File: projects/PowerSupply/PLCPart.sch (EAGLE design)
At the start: 31 parts, among them IC1 L7818CV, IC2 L7918CV, IC3 LM741P, IC4 LM741P, IC5 L7915CV, IC6 L7815CV, IC7 LM358N, IC8 LM358N, X1 MCU-PWR, X2 MCU-IN, X3 MCU-OUT

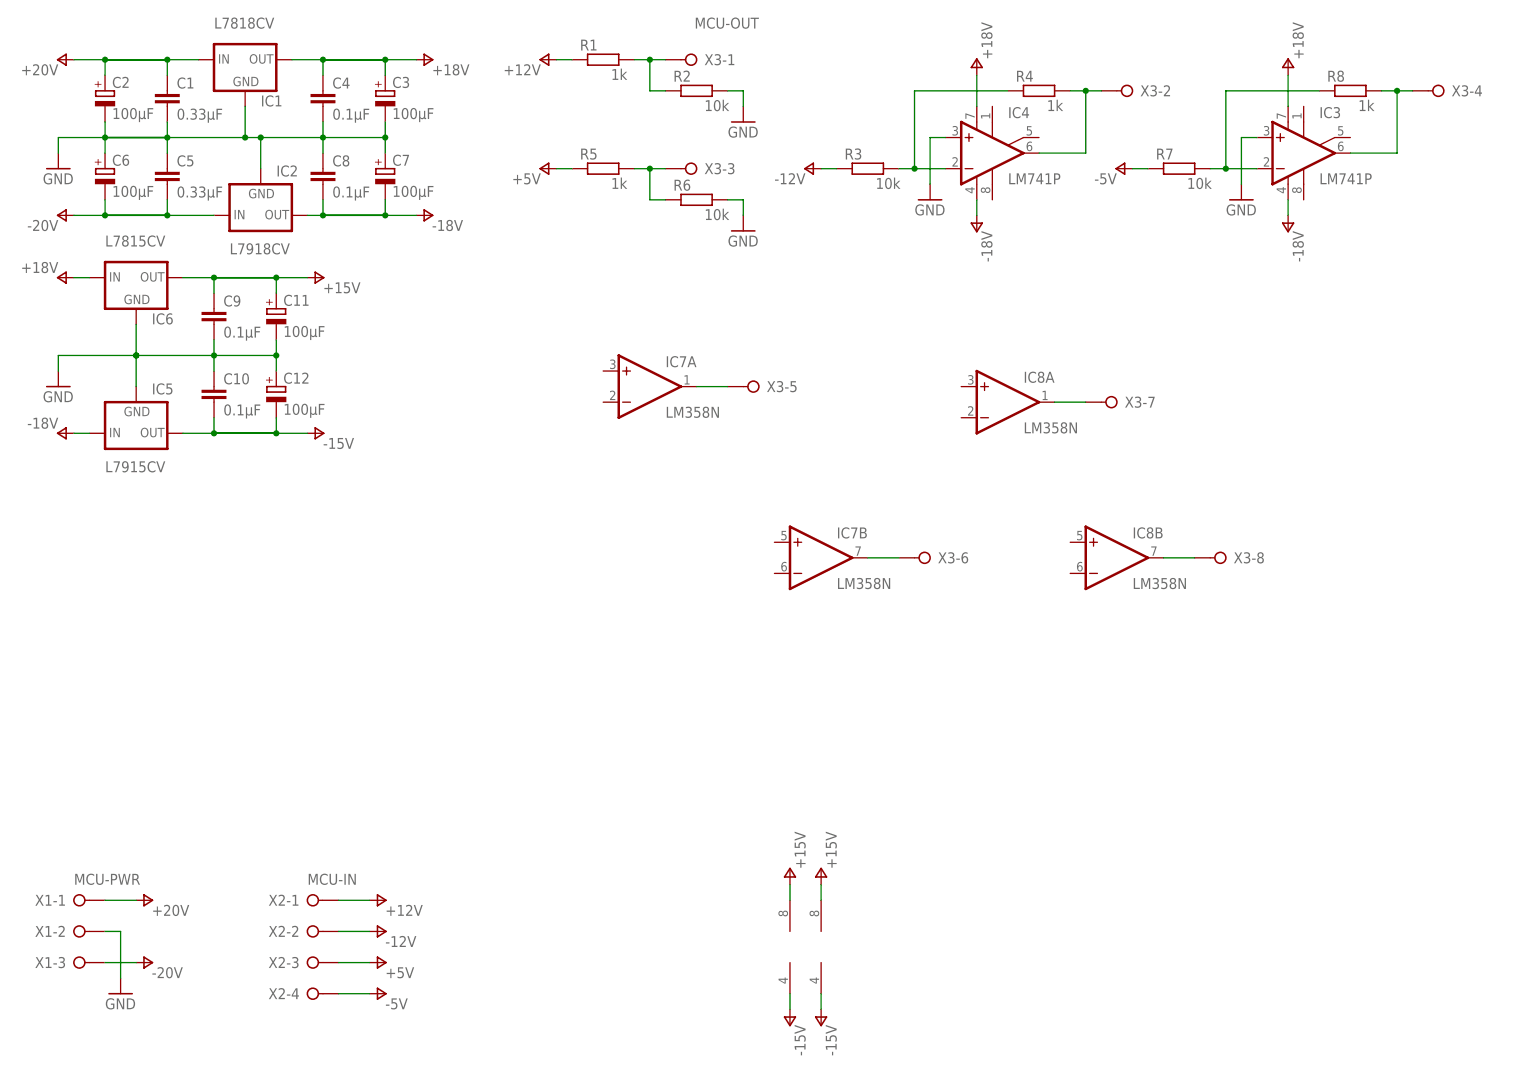
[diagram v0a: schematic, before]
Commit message: feat: plc part modified
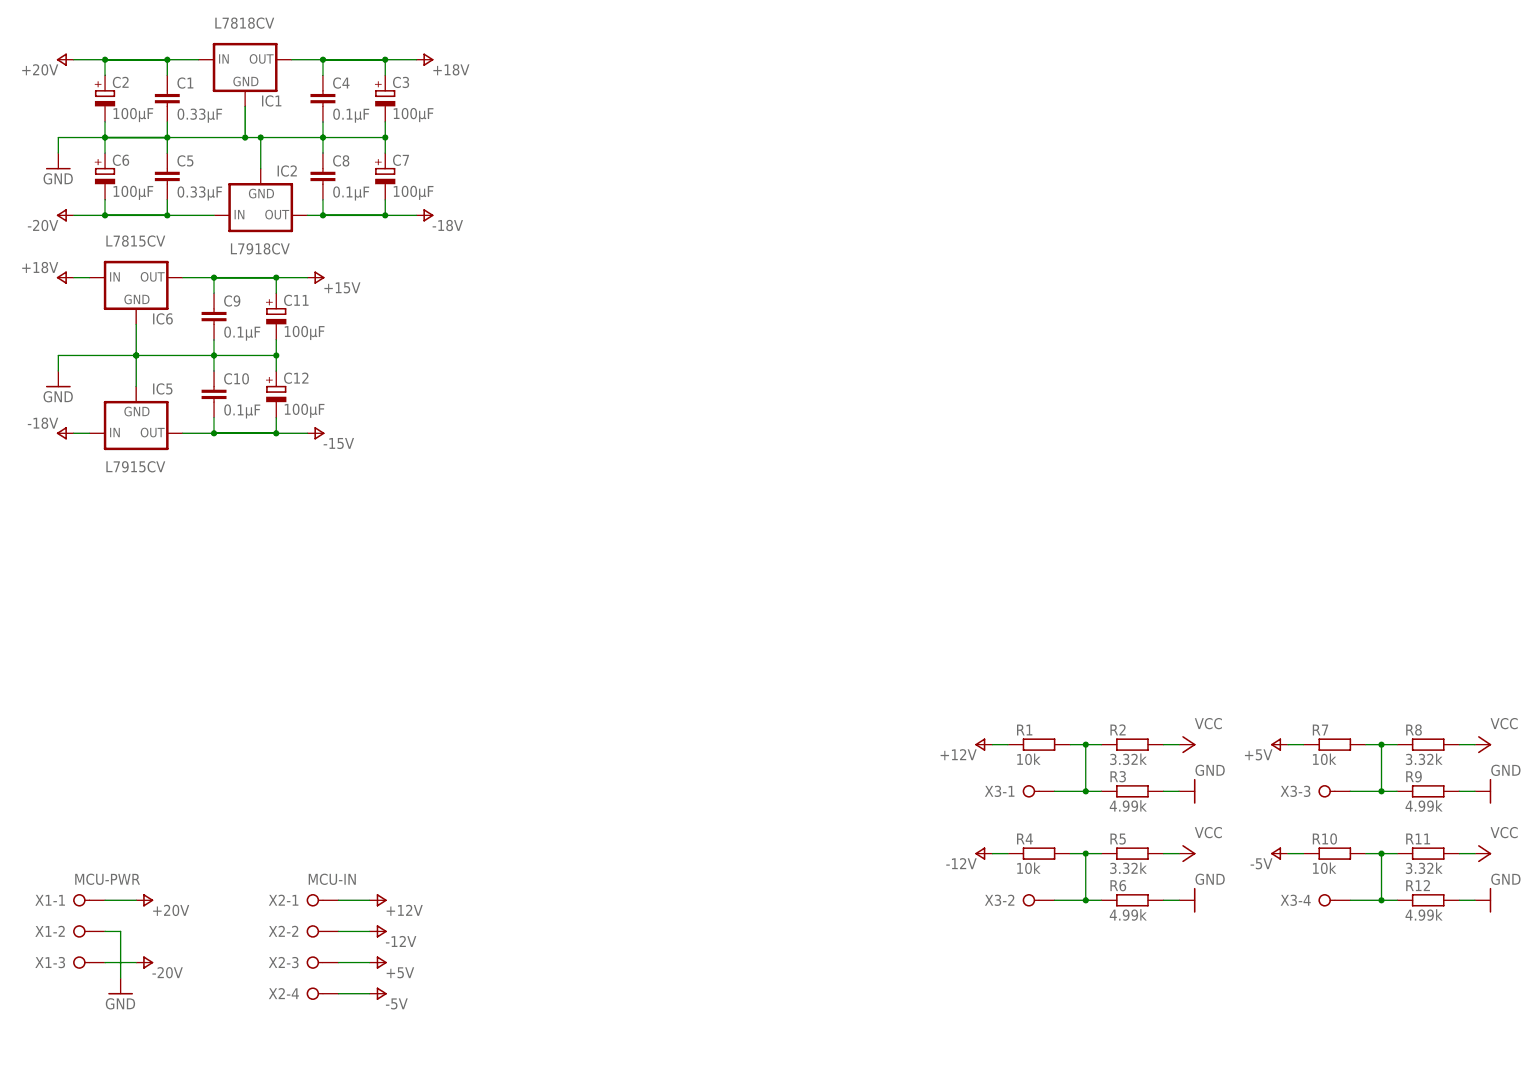
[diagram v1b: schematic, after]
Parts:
- removed IC3, IC4: LM741P, linear:LM741P
- removed IC7, IC8: LM358N, linear:LM358N
- added R10: 10k, rcl:R-EU_0207/10
- added R11: 3.32k, rcl:R-EU_0207/10
- added R12, R9: 4.99k, rcl:R-EU_0207/10
- R1, R4: value 1k -> 10k
- R2: value 10k -> 3.32k
- R3, R6: value 10k -> 4.99k
- R5, R8: value 1k -> 3.32k
- X3: value MCU-OUT -> (none); device con-wago-508:W237-08P -> con-wago-508:W237-04P
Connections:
- removed net N$10: IC8B.OUT, X3-8.KL
- removed net N$5: R5.2, R6.1, X3-3.KL
- removed net N$6: IC3.OUT, R8.2, X3-4.KL
- removed net N$7: IC7A.OUT, X3-5.KL
- removed net N$8: IC7B.OUT, X3-6.KL
- removed net N$9: IC8A.OUT, X3-7.KL
- new net VCC: R11.2, R2.2, R5.2, R8.2
- net +15V: no longer IC7P.V+, IC8P.V+
- net +18V: no longer IC3.V+, IC4.V+
- net +5V: now also R7.1; no longer R5.1
- net -12V: now also R4.1; no longer R3.1
- net -15V: no longer IC7P.V-, IC8P.V-
- net -18V: no longer IC3.V-, IC4.V-
- net -5V: now also R10.1; no longer R7.1
- net GND: now also R12.2, R3.2, R9.2; no longer IC3.+IN, IC4.+IN, R2.2
- net N$1: now also R1.2, R2.1, R3.1, X3-1.KL; no longer IC4.-IN, R3.2, R4.1
- net N$2: now also R5.1, R6.1; no longer IC4.OUT
- net N$3: now also R9.1, X3-3.KL; no longer IC3.-IN
- net N$4: now also R10.2, R11.1, R12.1, X3-4.KL; no longer R1.2, R2.1, X3-1.KL
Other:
- moved on the sheet: R1, R2, R3, R4, R5, R6, R7, R8, X3-1, X3-2, X3-3, X3-4
